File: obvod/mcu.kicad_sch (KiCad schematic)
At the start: 18 parts, among them U1 STM32H7A3VITx

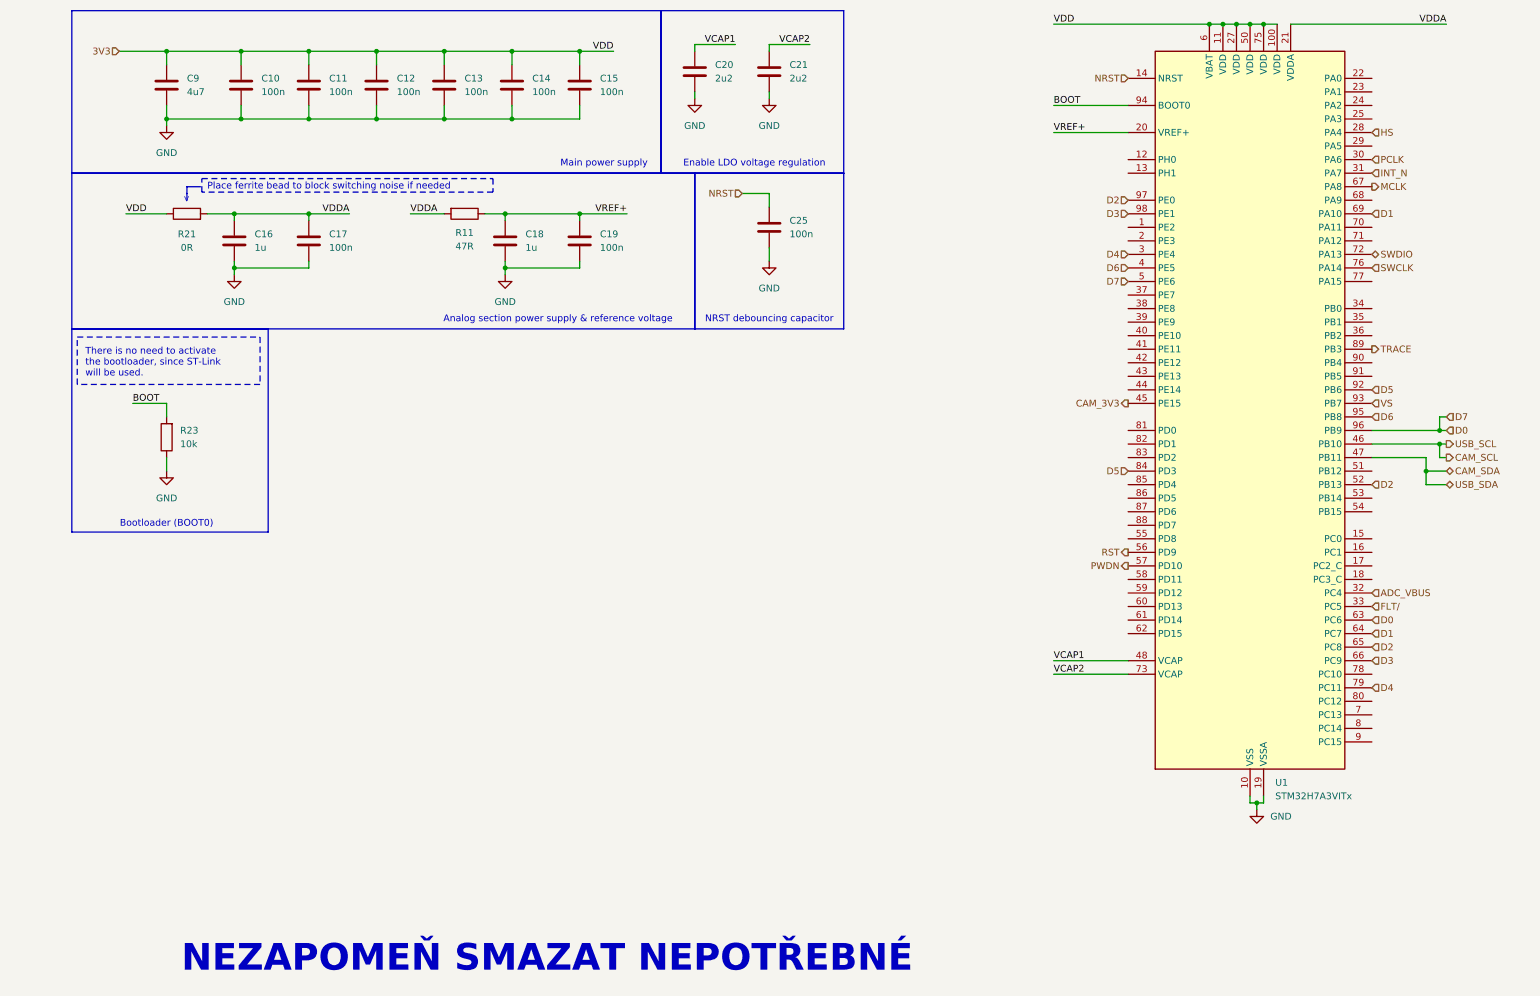
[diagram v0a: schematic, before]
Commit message: Crystal
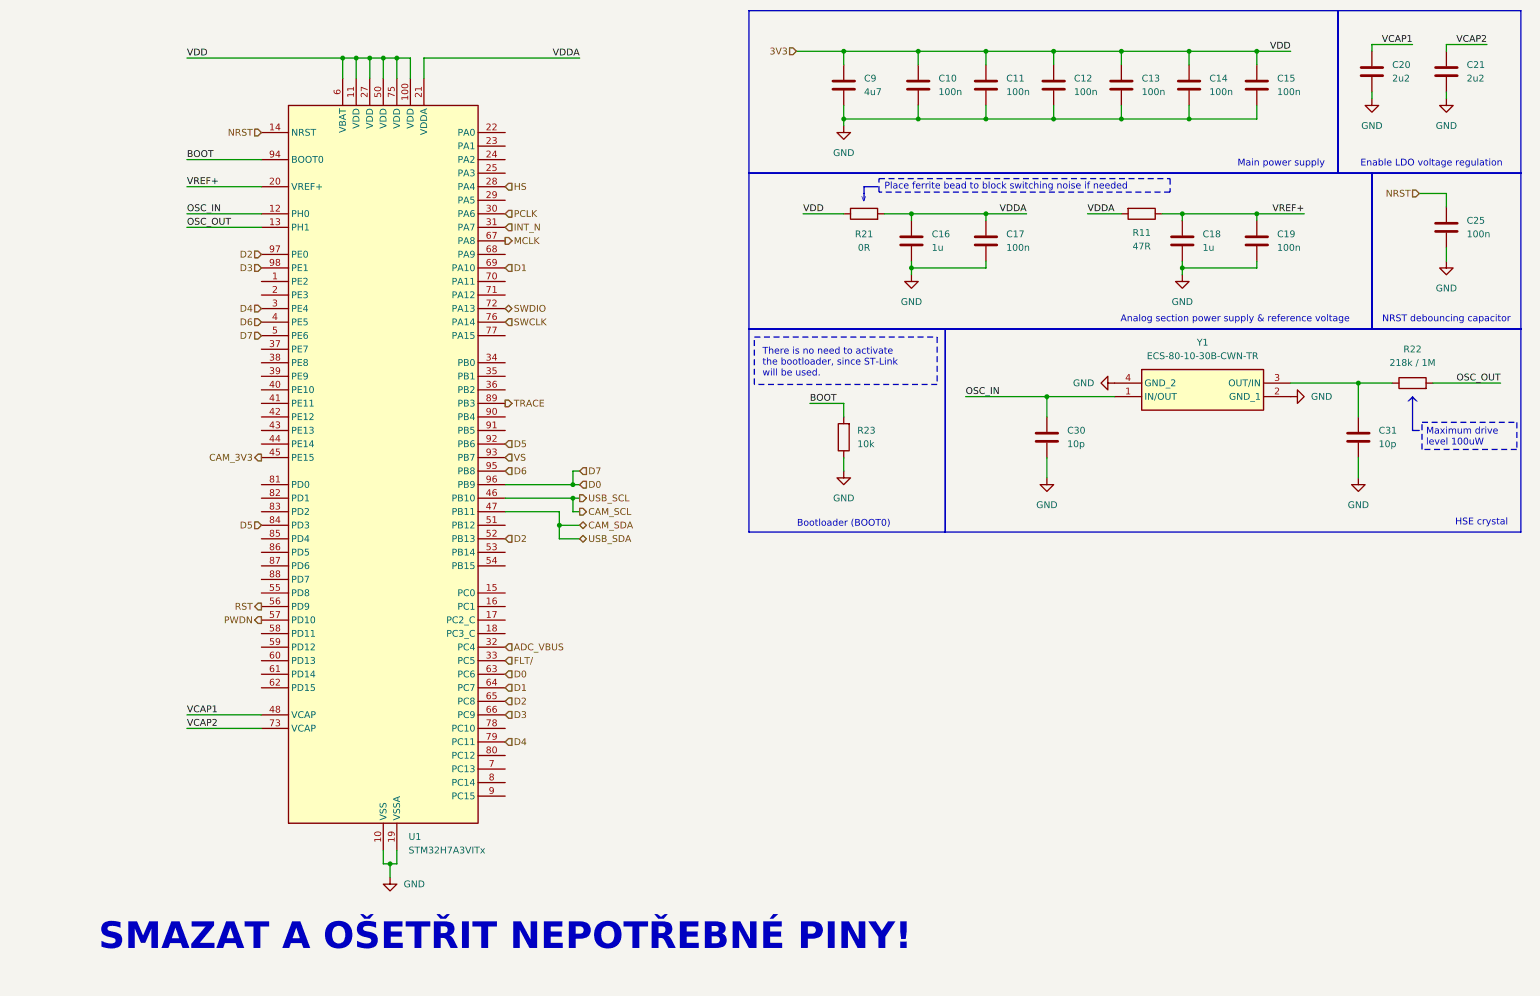
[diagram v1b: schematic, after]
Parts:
- added C30, C31: 10p, Capacitor_SMD:C_0402_1005Metric, symbol Device:C
- added R22: 218k / 1M, Resistor_SMD:R_0603_1608Metric, symbol Device:R
- added Y1: ECS-80-10-30B-CWN-TR, SamacSys_Parts:ECS801830BAGNTR, symbol SamacSys_Parts:ECS-80-10-30B-CWN-TR
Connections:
- net GND: now also C30.2, C31.2, Y1.2 (GND_1), Y1.4 (GND_2)
- net OSC_IN: now reaches U1.12 (PH0)
- net OSC_IN: now also C30.1, Y1.1 (IN/OUT)
- net OSC_OUT: now reaches U1.13 (PH1)
- net OSC_OUT: now also R22.2
- new net: C31.1, R22.1, Y1.3 (OUT/IN)
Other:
- note added: "HSE crystal"
- note added: "Maximum drive level 100uW"
- note added: "SMAZAT A OŠETŘIT NEPOTŘEBNÉ PINY!"
- note added: "^"
- note removed: "NEZAPOMEŇ SMAZAT NEPOTŘEBNÉ"
- moved on the sheet: C10, C11, C12, C13, C14, C15, C16, C17, C18, C19, C20, C21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
